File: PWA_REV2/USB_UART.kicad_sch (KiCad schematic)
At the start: 25 parts, among them J501 USB_C_Receptacle_USB2.0, Q205 MMBT2222A-7-F, U501 CH340B

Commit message: gerbers, generated and submitted files to PCPWAY to place an order, PWA_Rev, corrected and fixed the MPN and description of components.
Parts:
- U501: AssemblyType (none) -> SMT; Cost (none) -> 1.05; Distributor 1 (none) -> JLCPCB; Distributor 1 PN (none) -> C81010; MPN (none) -> CH340B
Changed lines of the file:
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@@
+      (effects (font (size 1.27 1.27)) hide)
+    )
+    (property "Cost" "1.05" (at 154.94 97.79 0)
+      (effects (font (size 1.27 1.27)) hide)
+    )
+    (property "Distributor 1" "JLCPCB" (at 154.94 97.79 0)
+      (effects (font (size 1.27 1.27)) hide)
+    )
+    (property "Distributor 1 PN" "C81010" (at 154.94 97.79 0)
+      (effects (font (size 1.27 1.27)) hide)
+    )
+    (property "AssemblyType" "SMT" (at 154.94 97.79 0)
+      (effects (font (size 1.27 1.27)) hide)
+    )
+    (property "Description" "2Mbps 3.3V Transceiver USB 2.0 SOP-16 USB Converters ROHS" (at 154.94 97.79 0)
+      (effects (font (size 1.27 1.27)) hide)
+    )
+    (property "MPN" "CH340B" (at 154.94 97.79 0)
       (effects (font (size 1.27 1.27)) hide)
     )

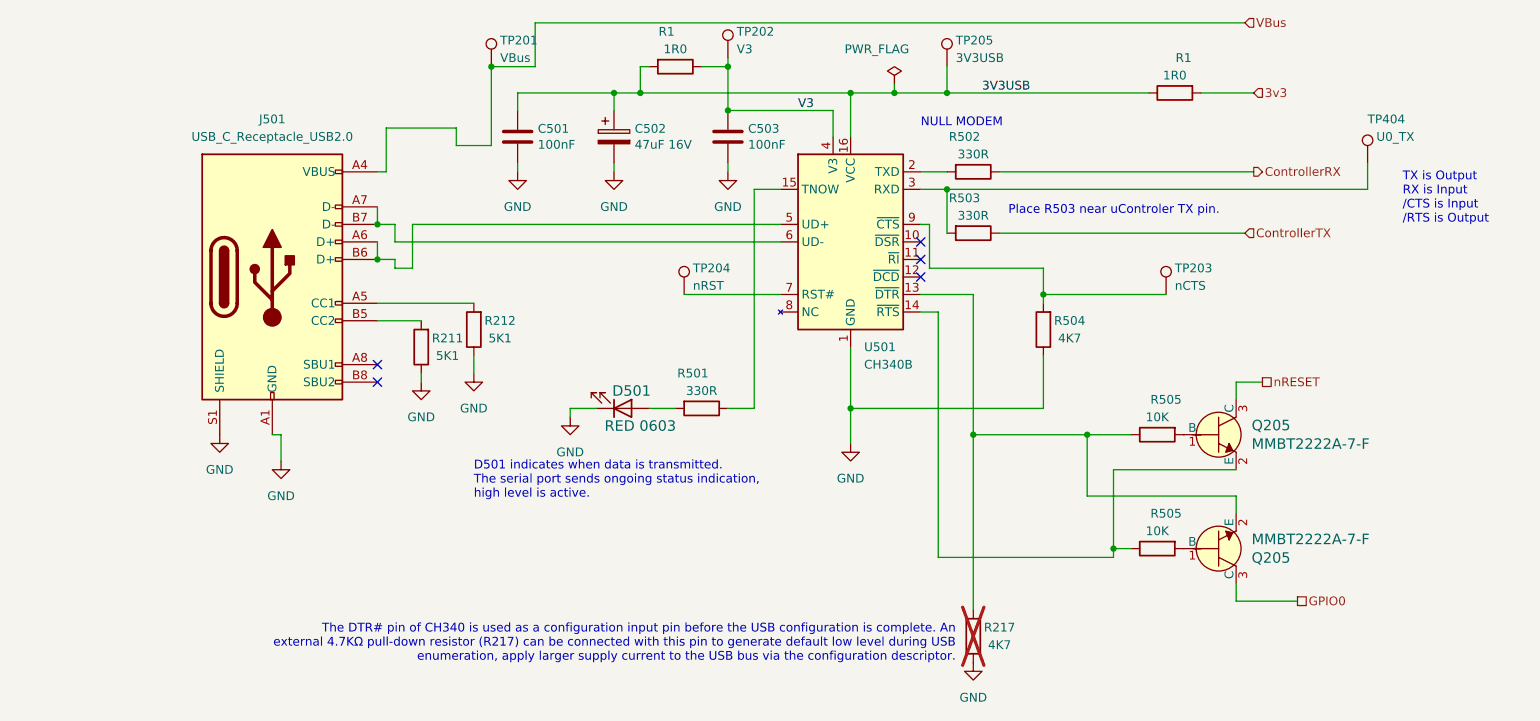
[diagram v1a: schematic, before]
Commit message: Hardware, PWA, Add a Jumper to BOM for J102 so that USB Connector Can Power Krake, issue 312.
:q
q
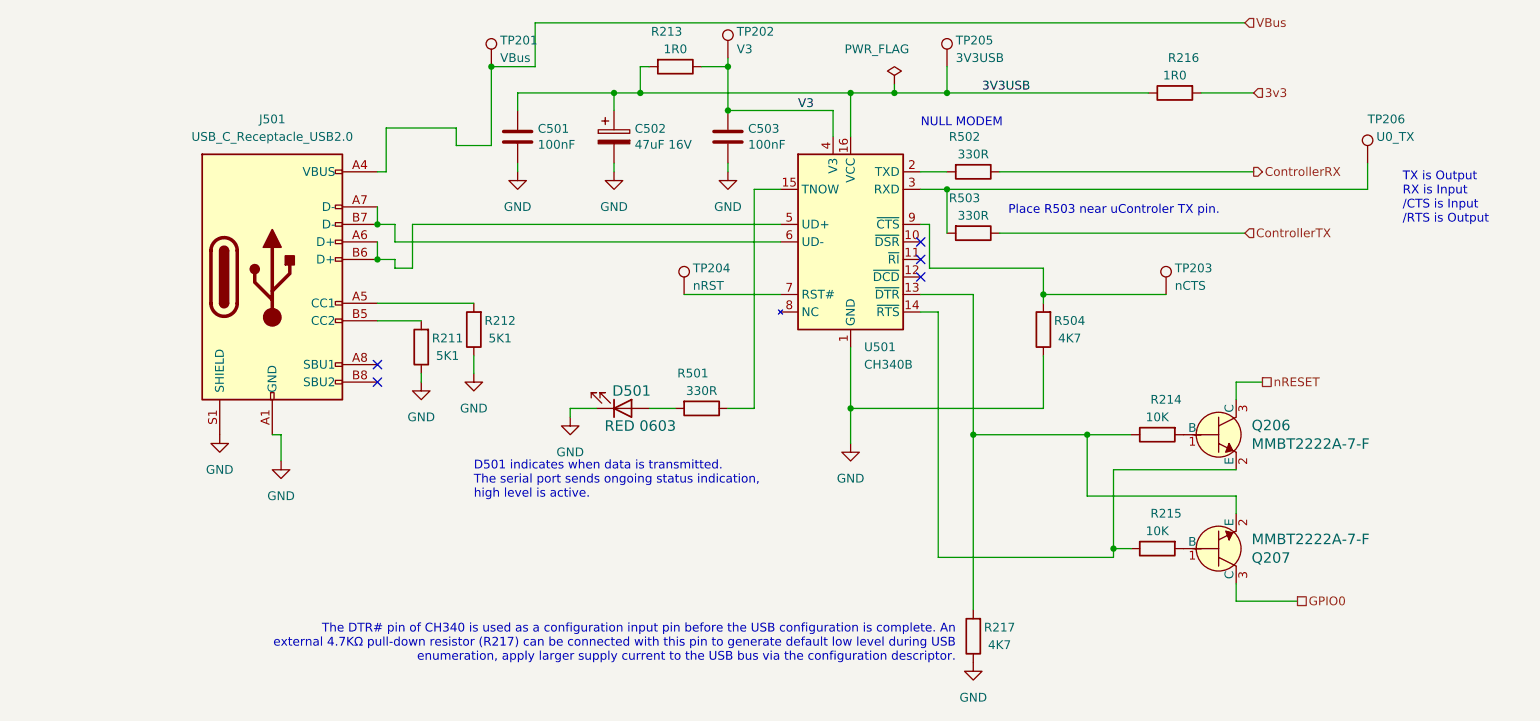
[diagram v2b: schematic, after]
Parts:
- R217: now fitted
- renumbered Q205 to Q206, Q205 to Q207, R1 to R213, R505 to R214, R505 to R215, R1 to R216, TP404 to TP206

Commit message: Revert "Hardware, PWA, Add a Jumper to BOM for J102 so that USB Connector Can Power Krake, issue 312."
This reverts commit c2819b8ee4999f733f52d823f88f6aefd6456fcc.
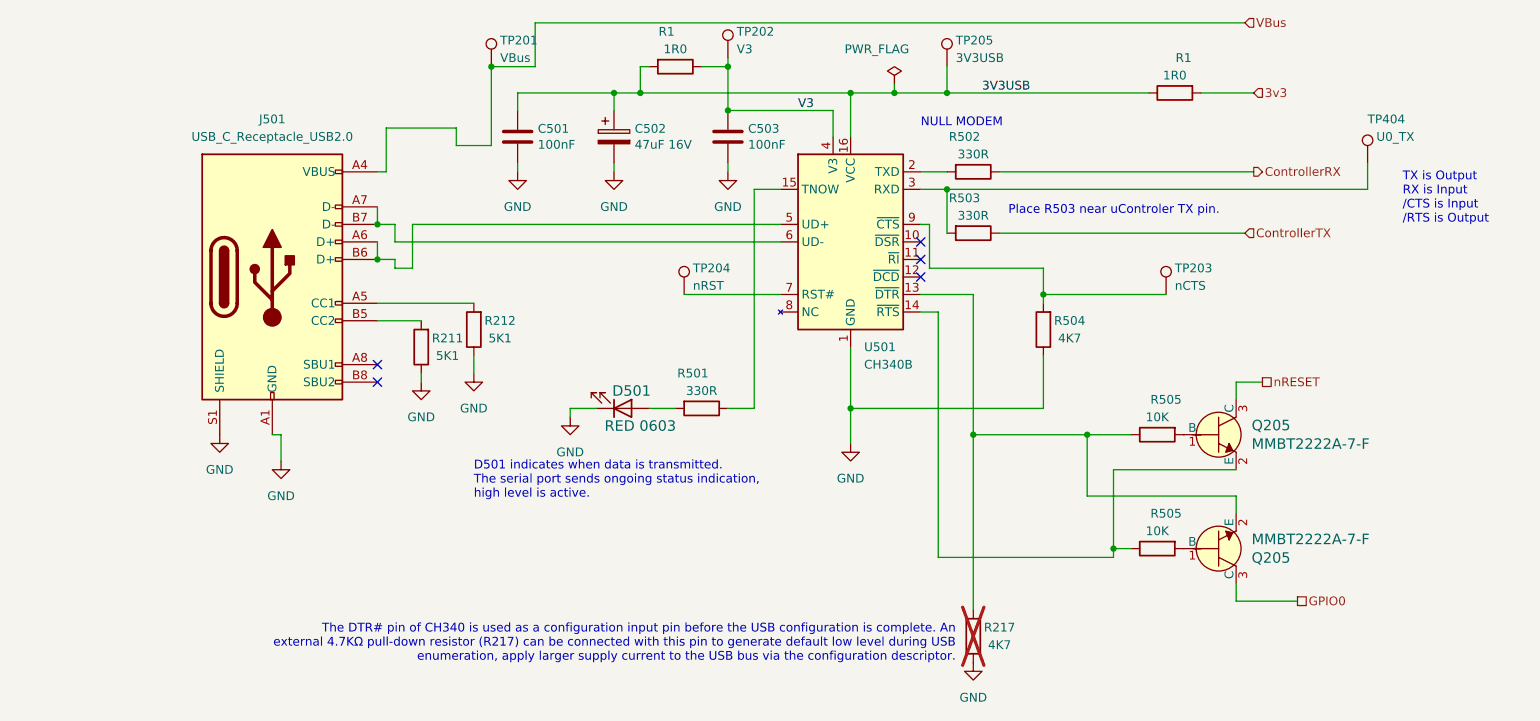
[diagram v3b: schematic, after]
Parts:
- R217: now not fitted
- renumbered Q206 to Q205, Q207 to Q205, R216 to R1, R213 to R1, R214 to R505, R215 to R505, TP206 to TP404
